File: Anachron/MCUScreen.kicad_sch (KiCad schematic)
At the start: 24 parts, among them J2 FFC2B35-18-G_REVA2, U3 ESP32-S3 N8R8, Y1 32.768kHz

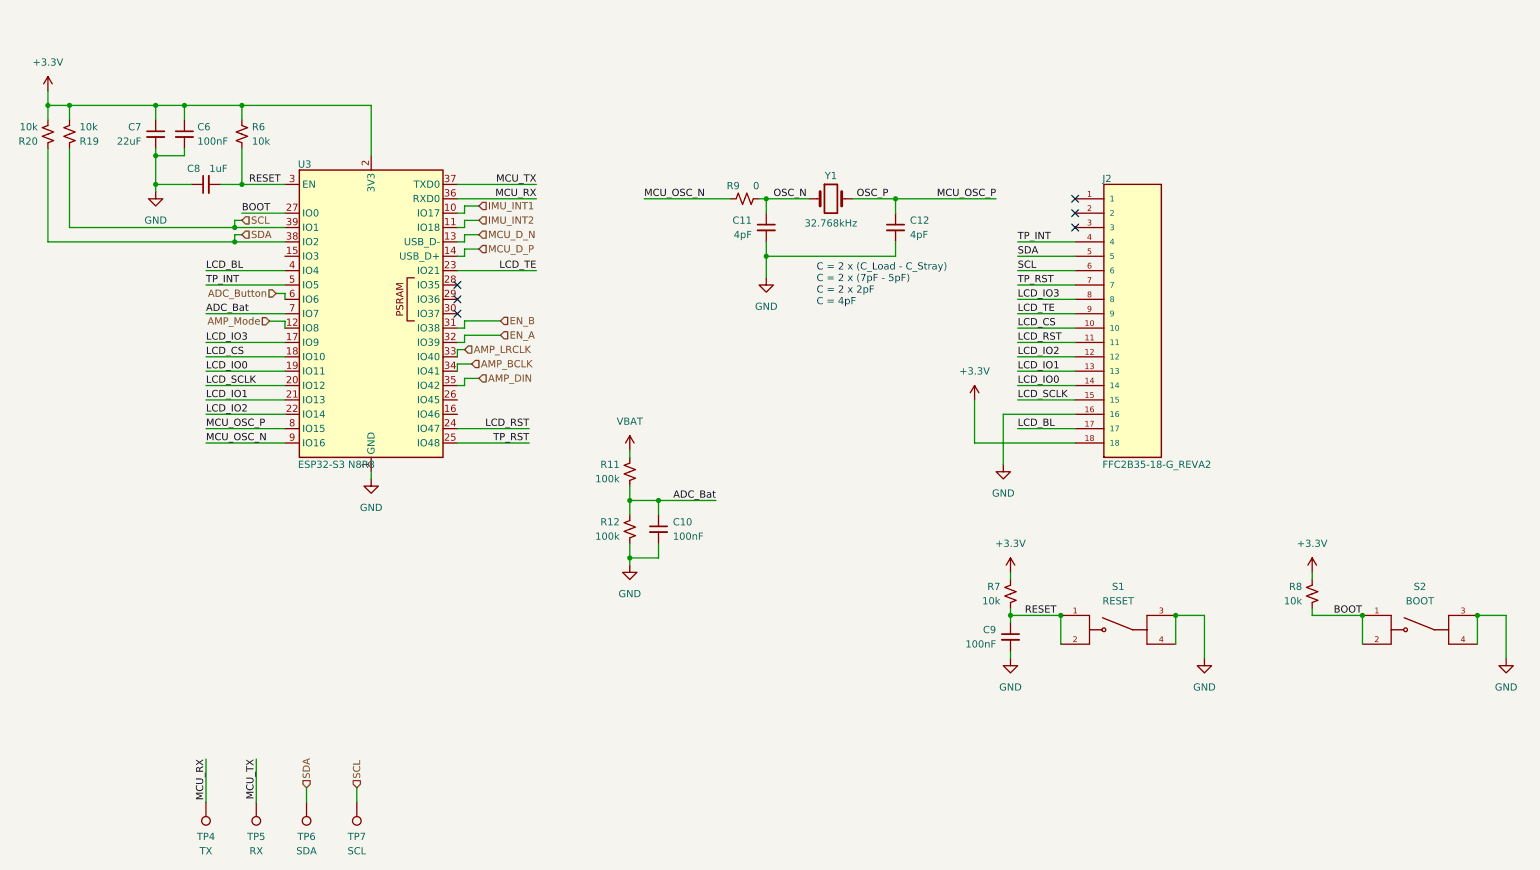
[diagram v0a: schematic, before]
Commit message: more changes!
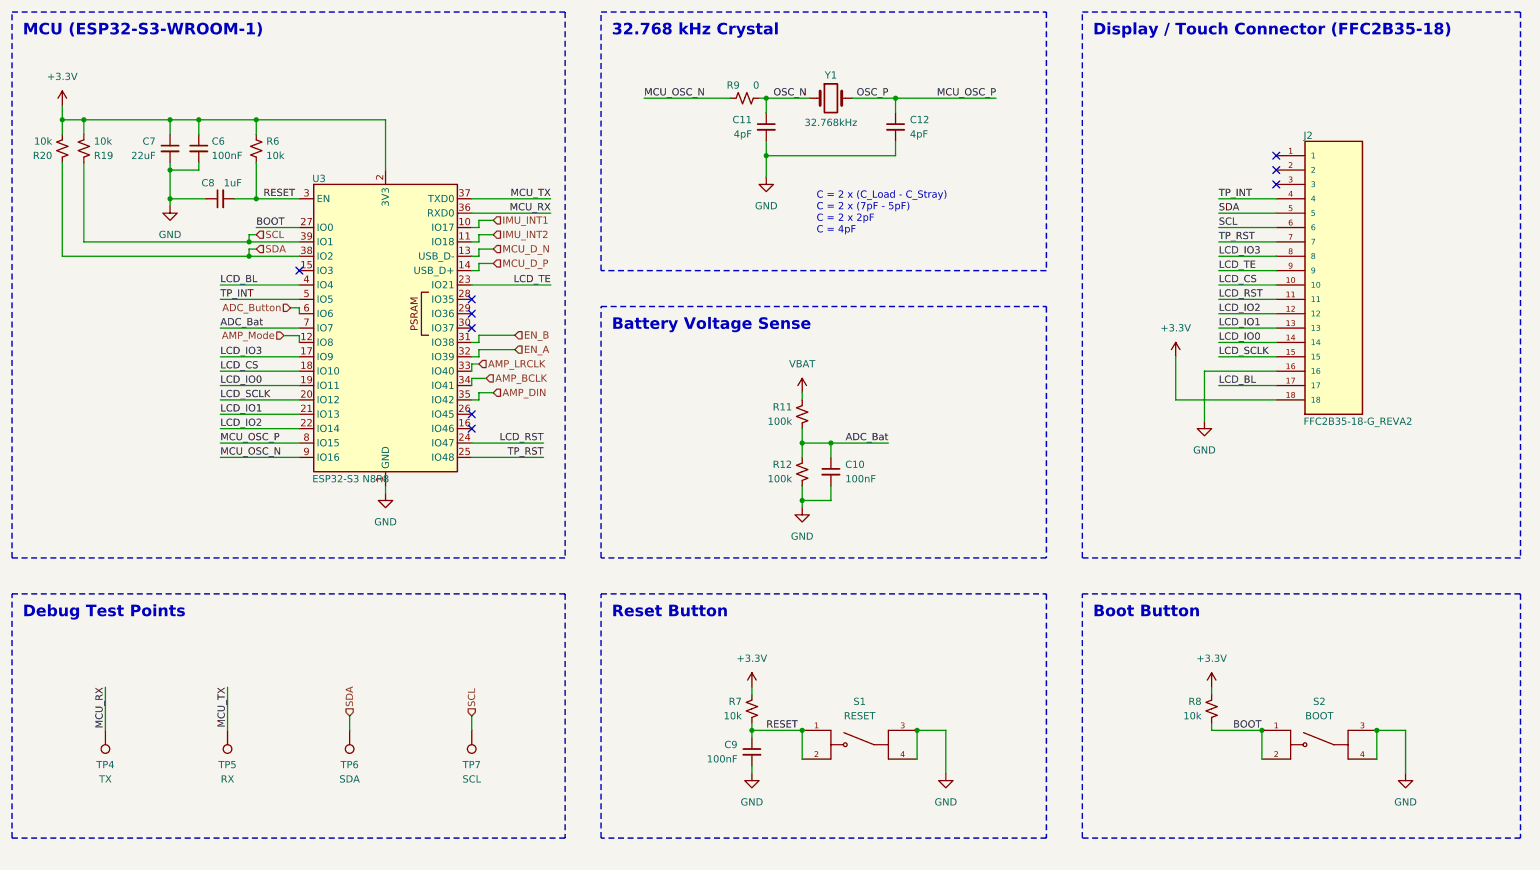
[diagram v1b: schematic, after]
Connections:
- no-connect marks 6 -> 9
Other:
- note added: "32.768 kHz Crystal"
- note added: "Battery Voltage Sense"
- note added: "Boot Button"
- note added: "Debug Test Points"
- note added: "Display / Touch Connector (FFC2B35-18)"
- note added: "MCU (ESP32-S3-WROOM-1)"
- note added: "Reset Button"
- moved on the sheet: C10, C11, C12, C6, C7, C8, C9, J2, R11, R12, R19, R20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
